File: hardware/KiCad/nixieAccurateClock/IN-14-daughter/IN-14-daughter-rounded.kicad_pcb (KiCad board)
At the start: 4 copper layers, 19 x 32 mm, 12 parts, among them J1 Conn_02x05_Odd_Even, U1 HV509K6-G

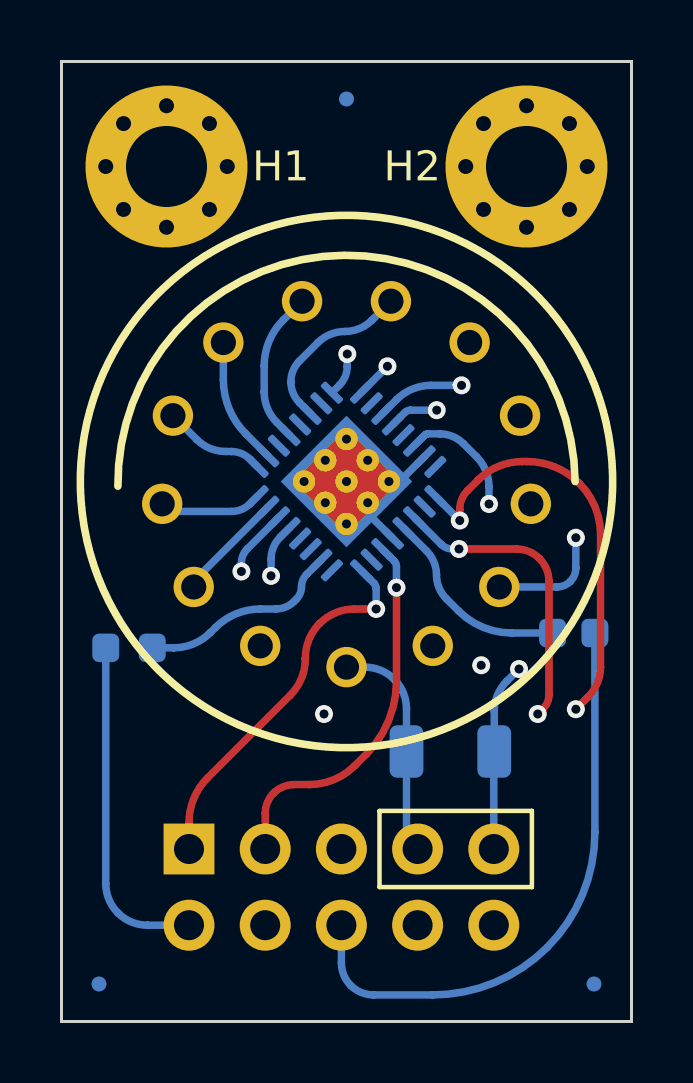
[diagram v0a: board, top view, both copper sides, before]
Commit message: add thermal reliefs
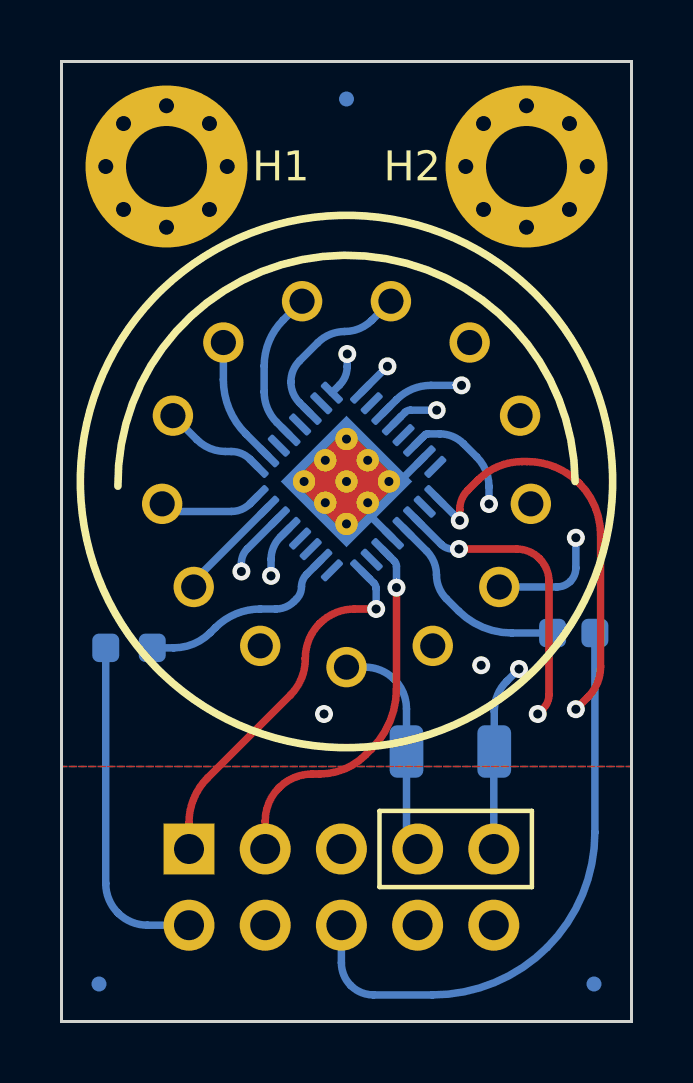
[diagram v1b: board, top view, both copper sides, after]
